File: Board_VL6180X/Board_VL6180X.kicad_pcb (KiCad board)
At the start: 2 copper layers, 20 x 16 mm, 11 parts, among them J1 Conn_01x06, U1 VL6180X

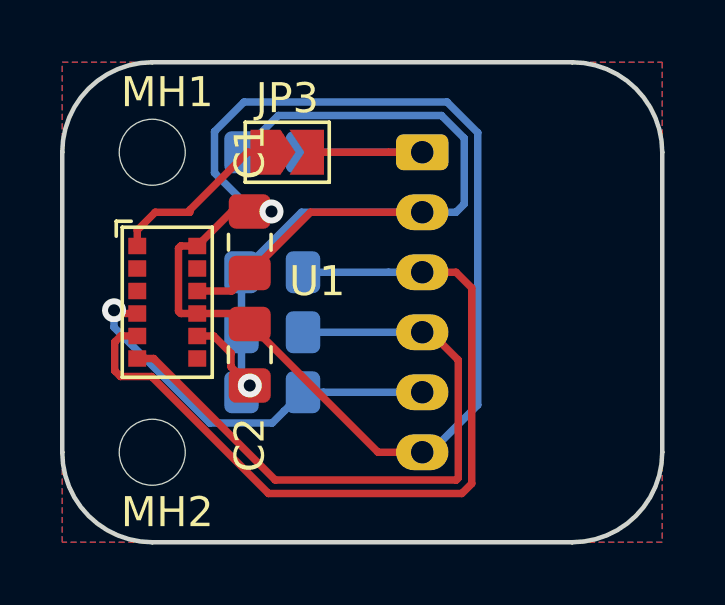
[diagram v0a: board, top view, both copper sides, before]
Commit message: update board
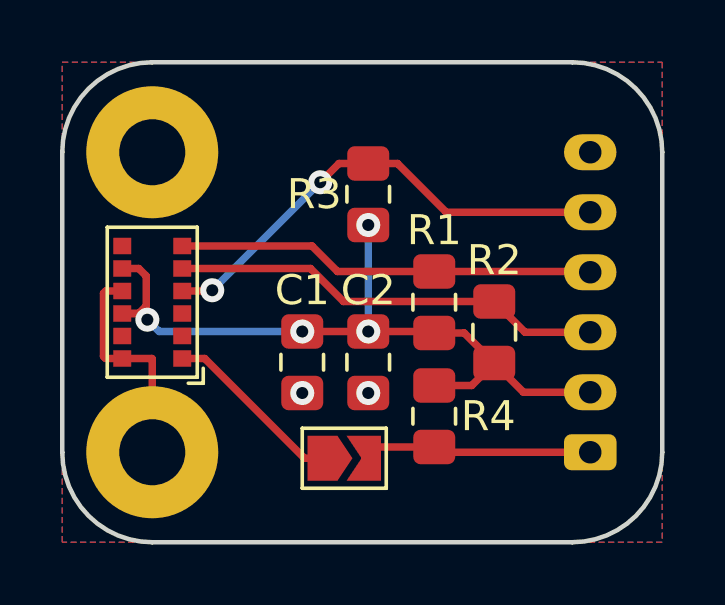
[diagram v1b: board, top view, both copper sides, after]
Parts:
- MH1, MH2: value MountingHole -> MountingHole_Pad; footprint MountingHole:MountingHole_2.2mm_M2 -> MountingHole:MountingHole_2.2mm_M2_Pad
- R1, R2, R3, R4: moved to F.Cu
- U1: footprint PhoenixRobotik:ST_LGA-12_2.8x4.8x1.0mm_P0.75mm -> PhenixRobotik:ST_LGA-12_2.8x4.8x1.0mm_P0.75mm
- moved J1 11.5 mm to (117.6, 93.0), turned to 90 degrees
- moved JP3 10.4 mm to (109.4, 93.2)
- moved R4 10.3 mm to (112.4, 91.8), turned to 270 degrees
- moved R2 7.67 mm to (114.4, 89.0), turned to 90 degrees
- moved R3 7.33 mm to (110.2, 84.4), turned to 90 degrees
- moved R1 5.49 mm to (112.4, 88.0), turned to 270 degrees
- moved C1 4.37 mm to (108.0, 90.0), turned to 270 degrees
- moved C2 3.96 mm to (110.2, 90.0), turned to 90 degrees
- moved U1 0.50 mm to (103.0, 88.0), turned to 180 degrees
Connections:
- MH1 pad 1: (no net) -> GND
- MH2 pad 1: (no net) -> GND
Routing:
- net GND: track 40.8 -> 7.53 mm, vias 1 -> 2
- net /I2C_SCL: track 27.9 -> 14.5 mm
- net +2V8: track 34.1 -> 25.4 mm, vias 1 -> 4
- net /I2C_SDA: track 21.9 -> 14.0 mm
- net /~XSHUT: track 13.4 -> 16.0 mm, vias 1 -> 2
